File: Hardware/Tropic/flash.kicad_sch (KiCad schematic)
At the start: 1 part, among them J4 53309-1070

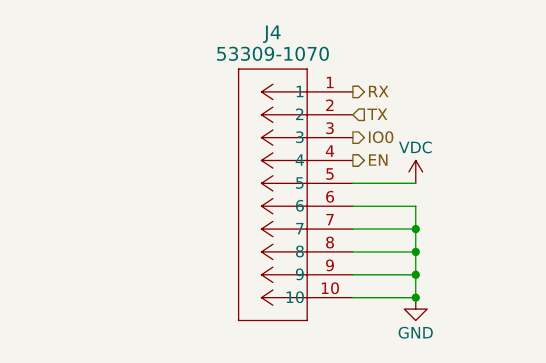
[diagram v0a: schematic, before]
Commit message: Rework on components
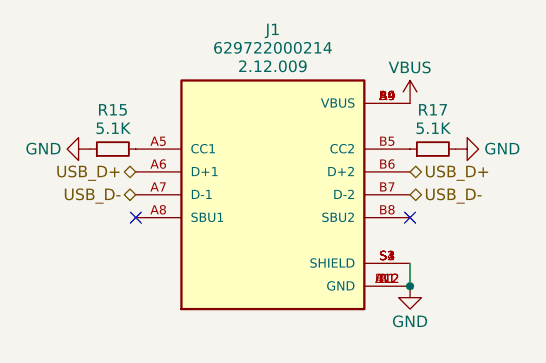
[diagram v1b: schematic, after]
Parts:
- removed J4: 53309-1070, manul_tech:CON_533091070, symbol manul_tech:53309-1070
- added J1: 629722000214, manul_tech:629722000214, symbol manul_tech:629722000214
- added R15, R17: 5.1K, Resistor_SMD:R_0402_1005Metric, symbol Device:R_Small
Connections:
- net GND: now also J1.A1 (GND), J1.A12 (GND), J1.B1 (GND), J1.B12 (GND), J1.S1 (SHIELD), J1.S2 (SHIELD), J1.S3 (SHIELD), J1.S4 (SHIELD), R15.1, R17.2
- new net: J1.A5 (CC1), R15.2
- new net: J1.B5 (CC2), R17.1
- new net USB_D+: J1.A6 (D+1), J1.B6 (D+2)
- new net USB_D-: J1.A7 (D-1), J1.B7 (D-2)
- new net VBUS: J1.A4 (VBUS), J1.A9 (VBUS), J1.B4 (VBUS), J1.B9 (VBUS)
- no-connect marks 0 -> 2
